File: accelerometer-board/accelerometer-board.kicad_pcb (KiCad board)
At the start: 2 copper layers, 25.4 x 19 mm, 23 parts, among them J1 Conn_01x08, J2 Conn_01x02, U1 LIS2HH12, U2 LIS2HH12, U3 FXMA2102L8X, U4 MCP1700T-2502E/TT

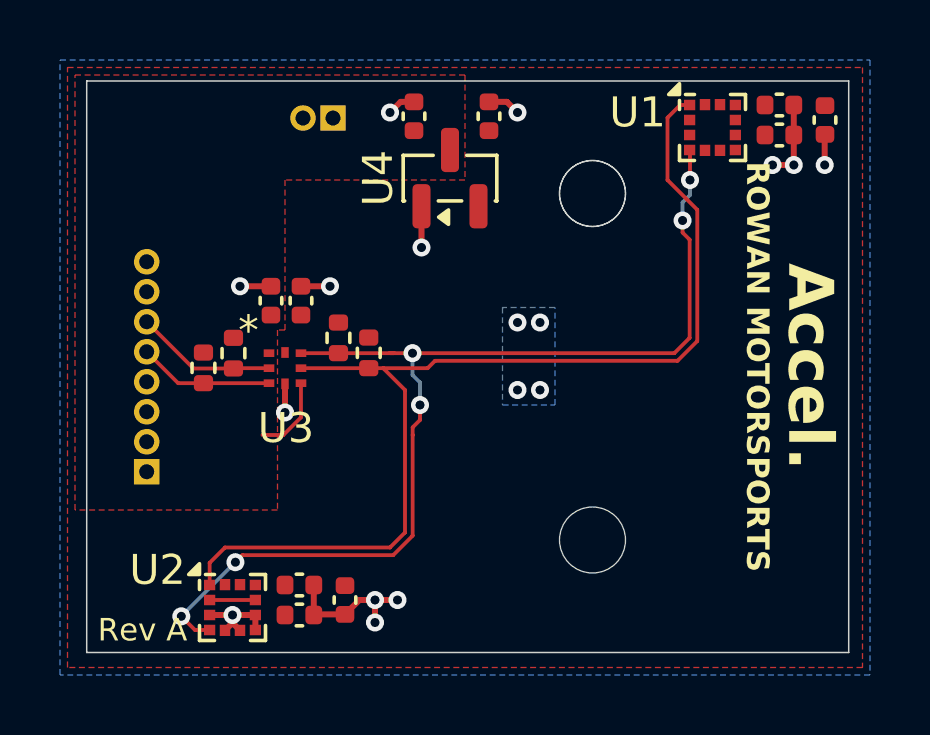
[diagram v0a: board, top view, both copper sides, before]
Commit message: accelerometer-board: Update to contain a single IMU chip
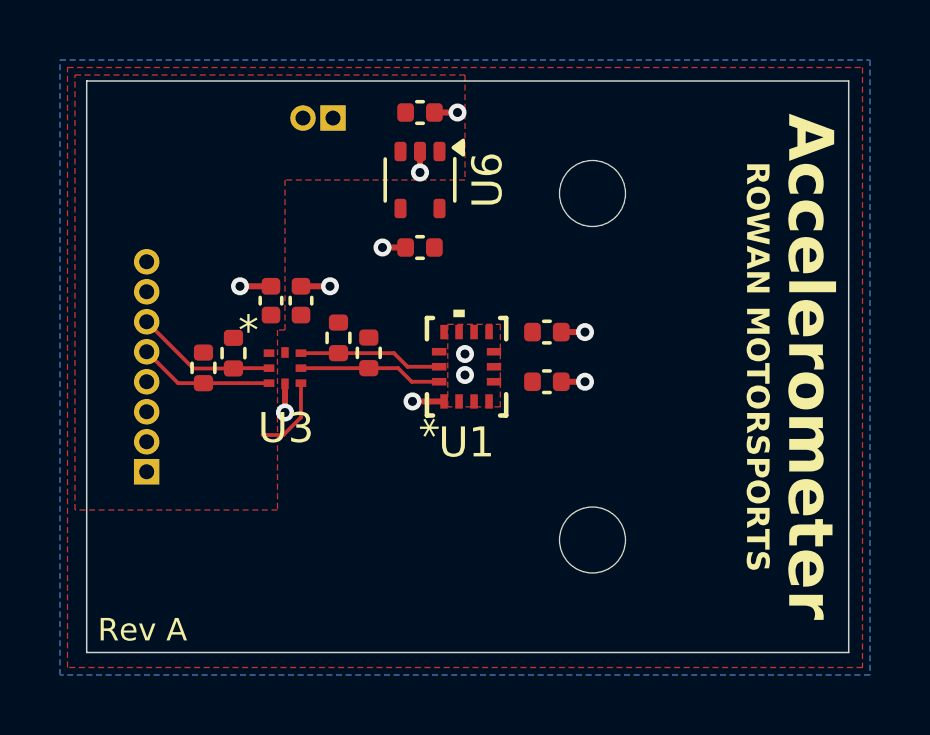
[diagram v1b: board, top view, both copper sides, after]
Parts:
- removed ?: , 
- removed C3, C5, C6: 100n, Capacitor_SMD:C_0402_1005Metric
- removed C4: 10u, Capacitor_SMD:C_0402_1005Metric
- removed U2: LIS2HH12, Package_LGA:LGA-12_2x2mm_P0.5mm
- removed U4: MCP1700T-2502E/TT, Package_TO_SOT_SMD:SOT-23
- added U6: MIC5365-3.3YC5-TR, Package_TO_SOT_SMD:SOT-353_SC-70-5, F.Cu at (97.8, 70.0)
- C1: value 10u -> 100n
- U1: value LIS2HH12 -> BMI323; footprint Package_LGA:LGA-12_2x2mm_P0.5mm -> BMI323:BMI323_BOS
- moved C1 11.7 mm to (102.0, 75.1), turned to 0 degrees
- moved U1 11.4 mm to (99.3, 76.2), turned to 90 degrees
- moved C2 11.3 mm to (102.0, 76.7)
- moved C10 4.94 mm to (97.8, 72.2), turned to 180 degrees
- moved C9 0.24 mm to (97.8, 67.8), turned to 0 degrees
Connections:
- C1 pad 1: +2V5 -> +3V3
- C10 pad 1: +2V5 -> +3V3
- C2 pad 1: +2V5 -> +3V3
- C8 pad 1: +2V5 -> +3V3
- J1 pad 5: /SCL_5V -> /SDA_5V
- J1 pad 6: /SDA_5V -> /SCL_5V
- R1 pad 1: +2V5 -> +3V3
- R1 pad 2: /SDA_2V5 -> /SCL_3V3
- R2 pad 1: +2V5 -> +3V3
- R2 pad 2: /SCL_2V5 -> /SDA_3V3
- R3 pad 2: /SDA_5V -> /SCL_5V
- R4 pad 2: /SCL_5V -> /SDA_5V
- U1 pad 1: /SCL_2V5 -> GND
- U1 pad 10: +2V5 -> unconnected-(U1-NC-Pad10)
- U1 pad 12: unconnected-(U1-INT1-Pad12) -> +3V3
- U1 pad 2: +2V5 -> unconnected-(U1-NC-Pad2)
- U1 pad 3: +2V5 -> unconnected-(U1-NC-Pad3)
- U1 pad 4: /SDA_2V5 -> unconnected-(U1-INT1-Pad4)
- U1 pad 5: GND -> +3V3
- U1 pad 8: GND -> +3V3
- U1 pad 9: +2V5 -> unconnected-(U1-INT2-Pad9)
- U3 pad 2: /SDA_5V -> /SCL_5V
- U3 pad 3: /SCL_5V -> /SDA_5V
- U3 pad 6: /SCL_2V5 -> /SDA_3V3
- U3 pad 7: /SDA_2V5 -> /SCL_3V3
- U3 pad 8: +2V5 -> +3V3
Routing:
- net /SDA_2V5: track 36.0 -> 0.00 mm, vias 6 -> 0
- net /SCL_2V5: track 35.8 -> 0.00 mm
- net GND: track 17.9 -> 7.83 mm, vias 13 -> 11
- net /SCL_3V3: track 0.00 -> 4.79 mm
- net /SDA_3V3: track 0.00 -> 4.79 mm
- net +2V5: track 1.53 -> 0.00 mm, vias 4 -> 0
- added copper zone on F.Cu, net +3V3
- added copper zone on F.Cu, net GND
- removed copper zone on B.Cu, net +2V5
- removed copper zone on F.Cu, net +2V5
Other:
- board text added: "Accelerometer"
- board text removed: "Accel."

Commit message: accelerometer-board: Expose x2 interrupt lines from IMU
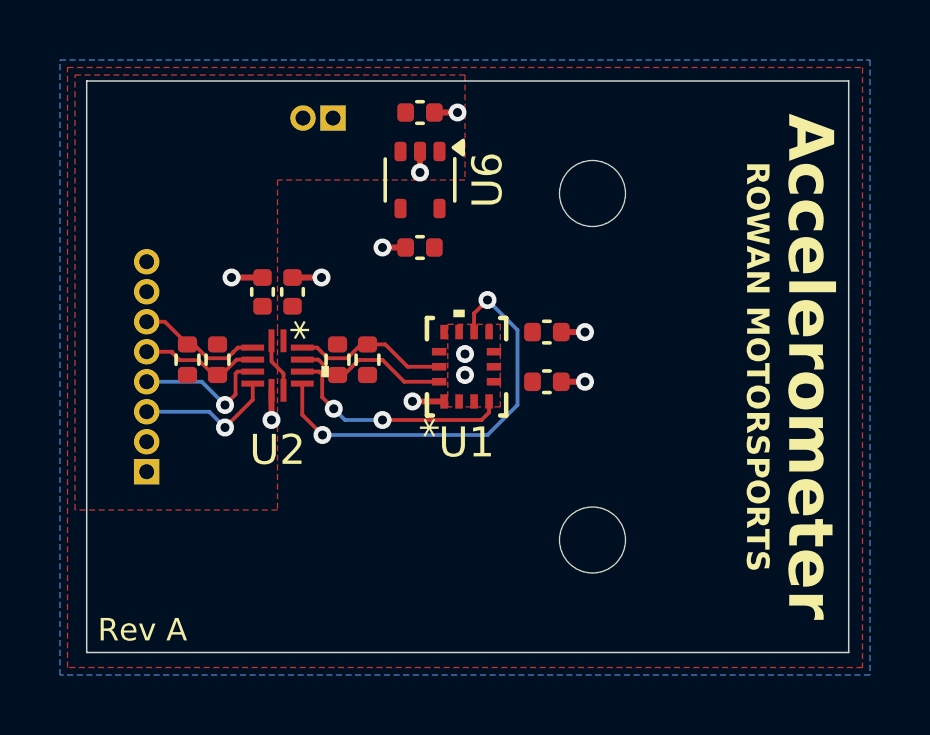
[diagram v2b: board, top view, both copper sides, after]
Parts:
- removed R1, R2, R3, R4: 4k7, Resistor_SMD:R_0402_1005Metric
- removed U3: FXMA2102L8X, FXMA2102L8X:MICROPAK8_1P6X1P6_ONS
- added R5: 4k7, Resistor_SMD:R_0402_1005Metric, F.Cu at (91.0, 76.0)
- added R6: 4k7, Resistor_SMD:R_0402_1005Metric, F.Cu at (90.0, 76.0)
- added R7: 4k7, Resistor_SMD:R_0402_1005Metric, F.Cu at (96.0, 76.0)
- added R8: 4k7, Resistor_SMD:R_0402_1005Metric, F.Cu at (95.0, 76.0)
- added U2: FXMAR2104UMX, FXMA2104L8X:ULTRATHIN_MLP_12L_ONS, F.Cu at (93.0, 76.2)
- moved C7 0.41 mm to (92.5, 73.7)
- moved C8 0.41 mm to (93.5, 73.7)
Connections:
- J1 pad 3: unconnected-(J1-Pin_3-Pad3) -> /IMU_INT2_5V
- J1 pad 4: unconnected-(J1-Pin_4-Pad4) -> /IMU_INT1_5V
- U1 pad 4: unconnected-(U1-INT1-Pad4) -> /IMU_INT1_3V3
- U1 pad 9: unconnected-(U1-INT2-Pad9) -> /IMU_INT2_3V3
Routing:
- net /IMU_INT2_3V3: track 0.00 -> 14.1 mm, vias 0 -> 2
- net /IMU_INT1_3V3: track 0.00 -> 7.81 mm, vias 0 -> 2
- net /IMU_INT1_5V: track 0.00 -> 4.72 mm, vias 0 -> 1
- net /IMU_INT2_5V: track 0.00 -> 4.67 mm, vias 0 -> 1
- net +5V: track 2.67 -> 1.82 mm
- net /SCL_5V: track 4.73 -> 4.19 mm
